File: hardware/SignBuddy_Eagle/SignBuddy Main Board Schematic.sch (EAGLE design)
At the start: 50 parts, among them U1 STM32L053C8T6D, U2 NCP115ASN330T2G

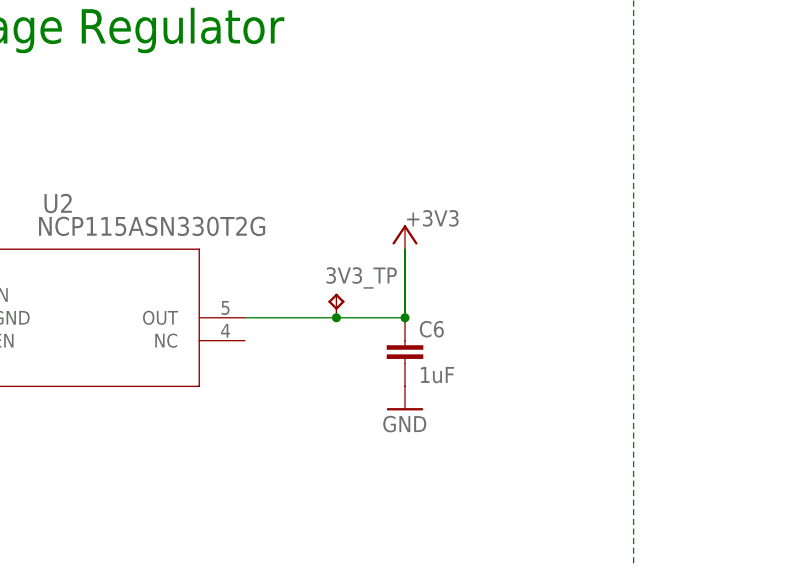
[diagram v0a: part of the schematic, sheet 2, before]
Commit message: small position adjustments
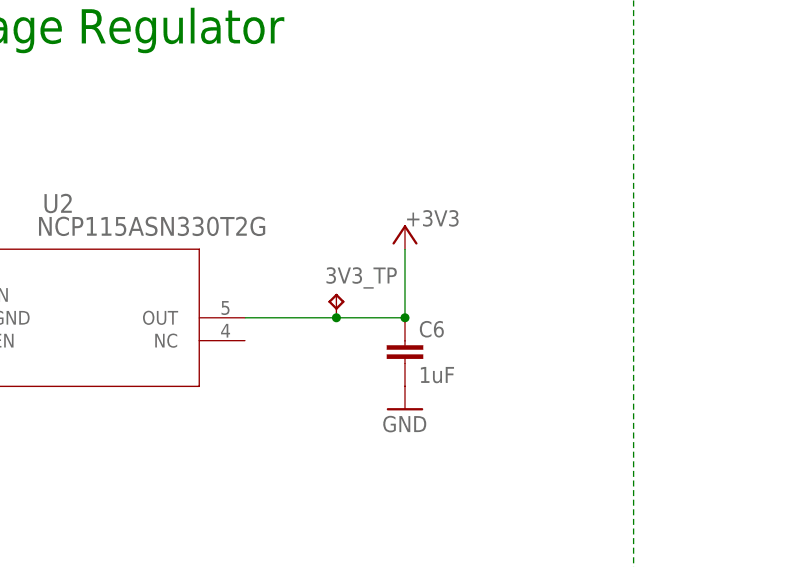
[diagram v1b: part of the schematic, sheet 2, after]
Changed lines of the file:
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@@
 <junction x="-35.56" y="48.26"/>
 <pinref part="+3V13" gate="G$1" pin="+3V3"/>
-<wire x1="-27.94" y1="48.26" x2="-27.94" y2="55.88" width="0.1524" layer="91"/>
 <junction x="-27.94" y="48.26"/>
 <wire x1="-27.94" y1="48.26" x2="-27.94" y2="55.88" width="0.1524" layer="91"/>
